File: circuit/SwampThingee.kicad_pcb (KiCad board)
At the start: 2 copper layers, 100 x 69 mm, 87 parts, among them J2 HOLE, J3 HOLE, J4 HOLE, J5 HOLE, Q1 IRFS52N15DTRLP, Q2 BC547, SW1 reset, SW10 4S, SW2 mute, SW3 HEAD/AD, SW9 6S, U1 LM2576T-ADJ, U2 LM1117-5.0, U3 MAX6457, U4 LM1117-3.3, U5 TPA3220, U6 CSR_DebugSmall, U7 CSR8645_MODULE

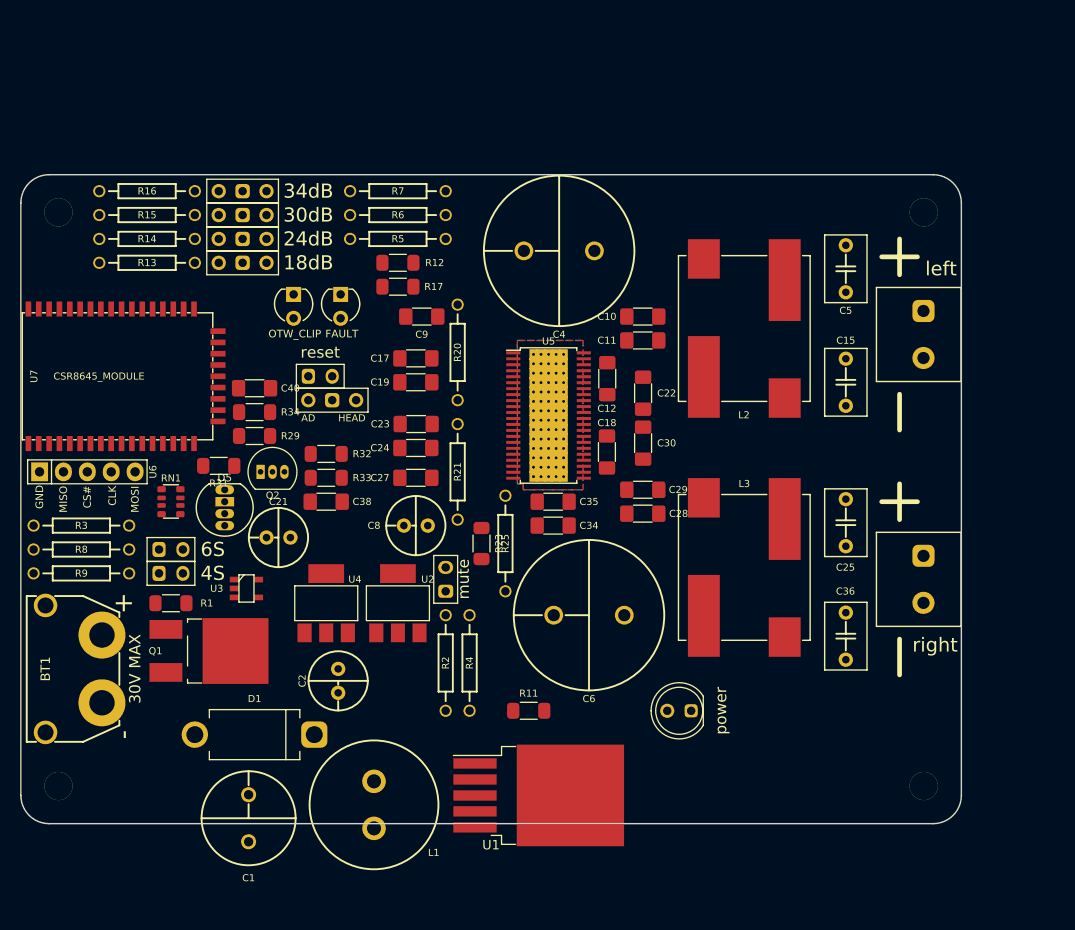
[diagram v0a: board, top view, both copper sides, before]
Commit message: narrow swamp thingee
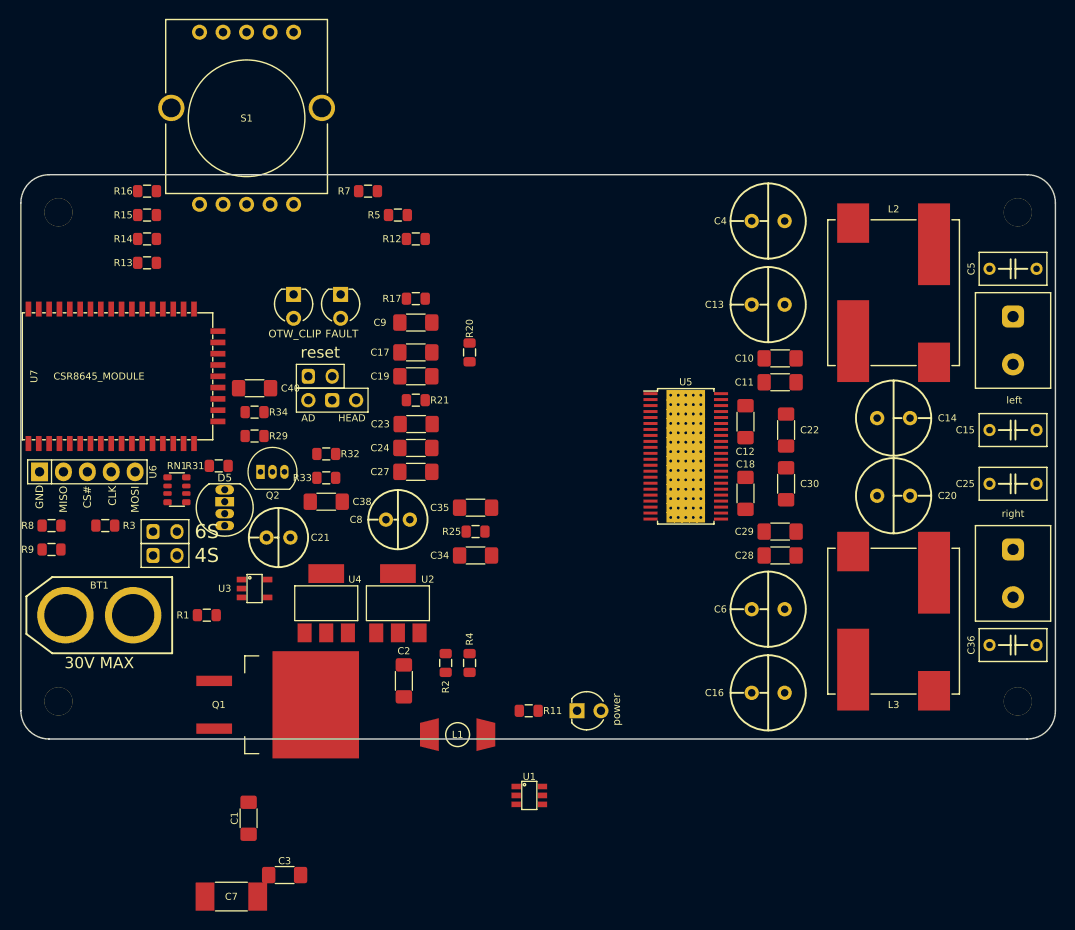
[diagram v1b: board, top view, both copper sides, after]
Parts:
- removed D1: 1N5822, NovaBox:DO-201AD_P12.70mm_Horizontal
- removed R23: 1K, NovaBox:R_1206
- removed R6: 100K, NovaBox:R_10MM
- removed S2: 18dB, NovaBox:JUMPER_3WAY
- removed S3: 24dB, NovaBox:JUMPER_3WAY
- removed S4: 30dB, NovaBox:JUMPER_3WAY
- removed S5: 34dB, NovaBox:JUMPER_3WAY
- removed SW2: mute, NovaBox:Switch_2.5mm
- added C13: 330μF, NovaBox:CPOL_D8_P3.5, F.Cu at (124.5, 43.8)
- added C14: 330μF, NovaBox:CPOL_D8_P3.5, F.Cu at (137.8, 55.9)
- added C16: 330μF, NovaBox:CPOL_D8_P3.5, F.Cu at (124.5, 85.1)
- added C20: 330μF, NovaBox:CPOL_D8_P3.5, F.Cu at (137.8, 64.1)
- added C3: 100nF, NovaBox:C_1206, F.Cu at (73.0, 104.5)
- added C7: 15μF, NovaBox:C_1812, F.Cu at (67.4, 106.8)
- added S1: GAIN_SEL, NovaBox:SR1712F-0204-20F0A-N9-N-027, F.Cu at (69.0, 24.0)
- BT1: footprint NovaBox:XT60PW-M -> NovaBox:XT60-M-NO_PM
- C1: value 100μF -> 100nF; footprint NovaBox:CPOL_D10_P4.5 -> NovaBox:C_1206
- C2: value 220μF -> 4.7μF; footprint NovaBox:CPOL_D6.3_P2.5 -> NovaBox:C_1206
- C4, C6: value 1000μF -> 330μF; footprint NovaBox:CPOL_D16_P7.5 -> NovaBox:CPOL_D8_P3.5
- D3: footprint NovaBox:LED_D5.0mm -> NovaBox:LED_D3.0mm
- L1: value 1500μH -> 68μH; footprint NovaBox:COILCRAFT_RFS1317 -> NovaBox:COIL_SRR6603
- Q1: footprint NovaBox:TO-252 -> NovaBox:TO-263-2
- R1, R11, R12, R17, R29, R31, R32, R33, R34: footprint NovaBox:R_1206 -> NovaBox:R_0805
- R13, R14, R15, R16, R20, R21, R5, R7: footprint NovaBox:R_10MM -> NovaBox:R_0805
- R2: value 7K5 -> 133K; footprint NovaBox:R_10MM -> NovaBox:R_0805
- R25: value 3R3 -> 3.3R; footprint NovaBox:R_10MM -> NovaBox:R_0805
- R3: value 16.9M -> 1.69M; footprint NovaBox:R_10MM -> NovaBox:R_0805
- R4: value 1K6 -> 22.1K; footprint NovaBox:R_10MM -> NovaBox:R_0805
- R8: value 1.05M -> 105K; footprint NovaBox:R_10MM -> NovaBox:R_0805
- R9: value 1.62M -> 162K; footprint NovaBox:R_10MM -> NovaBox:R_0805
- SPK1, SPK2: footprint NovaBox:SPKR_5MM -> NovaBox:SPKR_5MM_BLUE
- U1: value LM2576T-ADJ -> TPS560430; footprint NovaBox:TO-263-5_TabPin3 -> NovaBox:SOT-23-6
- moved C4 22.5 mm to (124.5, 34.9)
- moved C6 19.1 mm to (124.5, 76.2)
- moved C15 18.5 mm to (150.5, 57.1), turned to 0 degrees
- moved C25 18.3 mm to (150.5, 62.9), turned to 180 degrees
- moved C36 17.8 mm to (150.5, 80.0), turned to 180 degrees
- moved C5 17.8 mm to (150.5, 40.0), turned to 0 degrees
- moved L3 16.9 mm to (137.8, 77.5)
- moved L2 16.3 mm to (137.8, 42.5)
- moved C30 15.8 mm to (126.4, 62.9)
- moved C22 15.7 mm to (126.4, 57.1)
- moved C12 15.4 mm to (122.0, 56.3)
- moved C18 15.4 mm to (122.0, 63.9)
- moved C10 15.3 mm to (125.7, 49.5)
- moved C11 15.3 mm to (125.7, 52.1)
- moved C28 15.3 mm to (125.7, 70.5)
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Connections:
- C1 pad 1: +BATT -> Net-(C1-Pad1)
- C1 pad 2: GND -> Net-(C1-Pad2)
- C2 pad 1: +7.5V -> GND
- C2 pad 2: GND -> Net-(C2-Pad2)
- L1 pad 1: Net-(D1-Pad1) -> Net-(C1-Pad1)
- U1 pad 1: +BATT -> Net-(C1-Pad2)
- U1 pad 2: Net-(D1-Pad1) -> GND
- U1 pad 3: GND -> Net-(R2-Pad2)
- U1 pad 4: Net-(R2-Pad2) -> Net-(C2-Pad2)
- U1 pad 5: GND -> Net-(C2-Pad2)
- U5 pad 2: Net-(S2-Pad2) -> /GAIN_SLV
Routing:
- removed copper zone on B.Cu, net GND
- removed copper zone on F.Cu, net GND
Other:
- board size 100 x 69 mm -> 110 x 60 mm
